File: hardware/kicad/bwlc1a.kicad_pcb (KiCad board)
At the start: 4 copper layers, 80.5 x 50 mm, 177 parts, among them J1 USB_C_Receptacle_USB2.0, J2 JST-2PH, J3 JTAG_10PIN, J4 SMN-304, J5 BWIPX-1-001E, J6 Qwiic, J7 BWIPX-1-001E, Q2 PMV32UP, Q3 S8050, Q4 S8050, Q5 PMBT3904, Q6 PMBT3904, Q7 DMG1012UW, Q8 AO3407A, SW1 RESET, SW2 BOOT, U1 USBLC6-2SC6, U10 TPS7A0328DBVR, U11 TXB0106PWR, U12 TPS7A0333DBVR, U2 MCP73831-2-OT, U3 RT9080-33GJ5, U4 LSM6DSOTR, U5 MAX17048G+, U6 ESP32-S3-MINI-1, U7 L76L-M33, U8 SY8089A1AAC, U9 A7670C_24x24mm, Y1 32.768 kHz

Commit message: change teapotlabs logo library
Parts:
- G***: footprint Teapot:TeapotLogo -> bwlc1a:TeapotLogo
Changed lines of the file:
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@@
 		)
 	)
-	(footprint "Teapot:TeapotLogo"
+	(footprint "bwlc1a:TeapotLogo"
 		(layer "F.Cu")
 		(at 183.837 119.126)

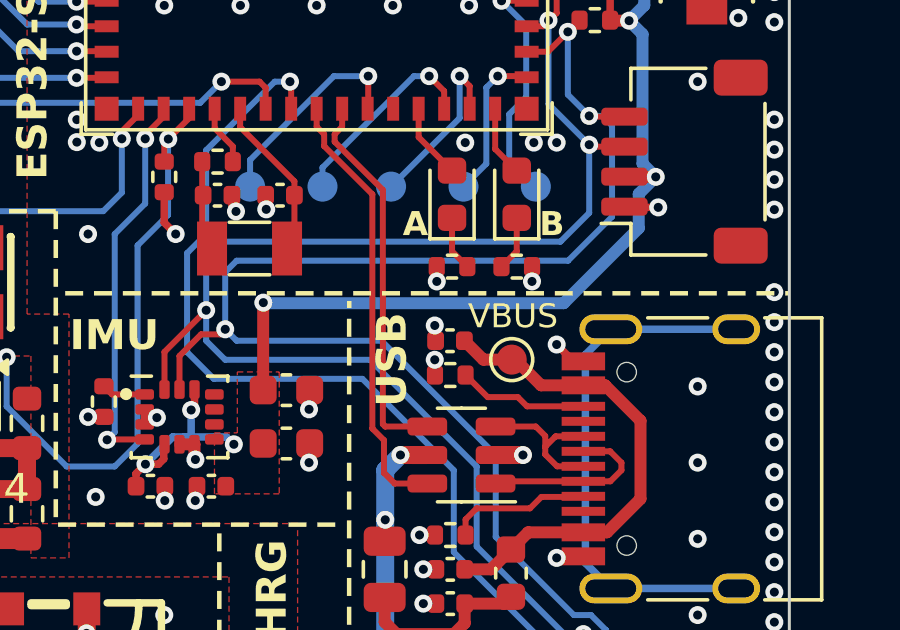
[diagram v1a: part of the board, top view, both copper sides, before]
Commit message: update schematics bom
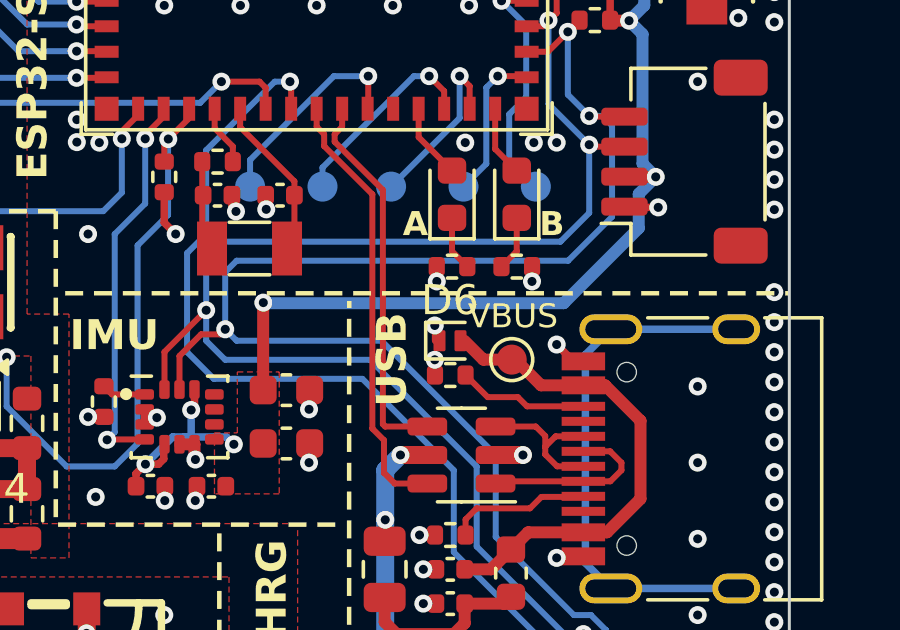
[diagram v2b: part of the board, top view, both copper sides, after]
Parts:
- D1: value Orange -> E6C0603SEAC1UDA
- D6: footprint Capacitor_SMD:C_0402_1005Metric -> Diode_SMD:D_SOD-882
- F1: value 0.75A -> SMD0805P075TF
- J2: footprint Teapot:JST_PH_S2B-PH-SM4-TB_1x02-1MP_P2.00mm_Horizontal -> bwlc1a:JST_PH_S2B-PH-SM4-TB_1x02-1MP_P2.00mm_Horizontal
- R3: value 1k -> 2k
